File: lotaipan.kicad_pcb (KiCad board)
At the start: 4 copper layers, 71 parts, among them J1 SMA_through, J2 SMA_through, P1 47309-2651_uSD_slot, P2 CONN_01X20, P3 CONN_01X25, P4 USB_OTG, Q1 MOS_N_SGD, U1 RN2483, U2 STM32F405R, U3 MCP1703, U4 MCP73831-2ACI/0T, U5 MIC94091YC6, U6 MIC94091YC6, Y1 12MHz, Y2 32kHz

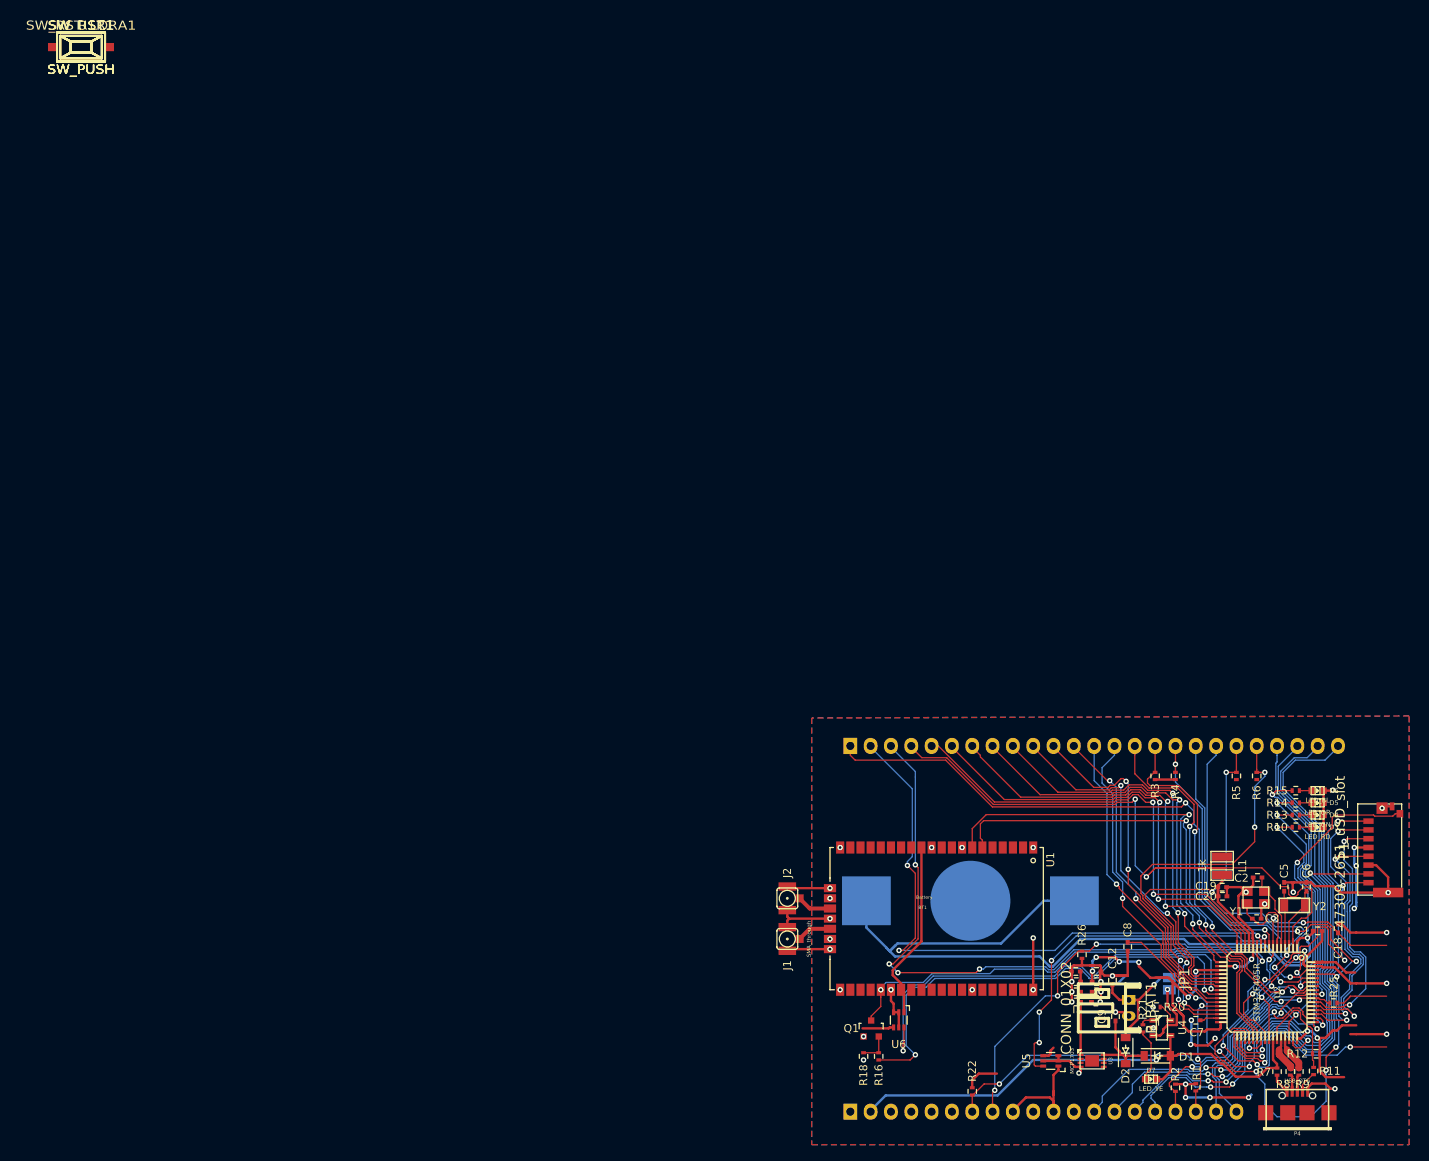
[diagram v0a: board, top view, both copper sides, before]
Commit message: Fixes and images
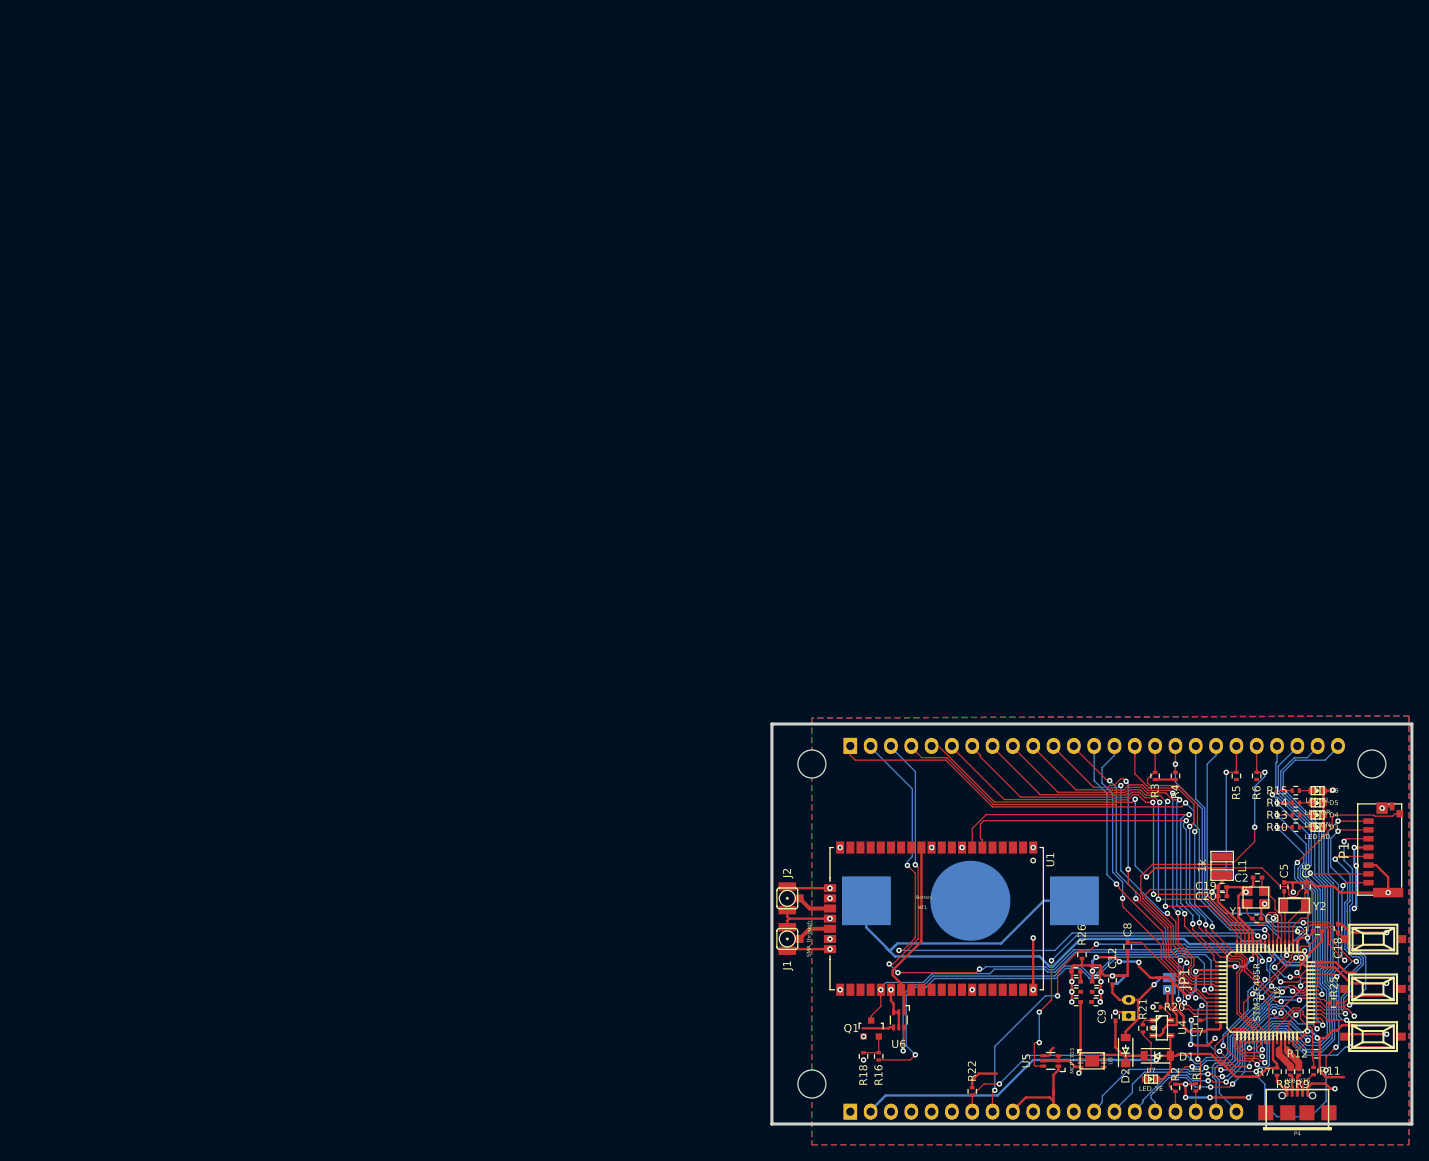
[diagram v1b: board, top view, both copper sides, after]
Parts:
- added REF**: EuroBoard_viertel_Type-I_80mmX50mm_holes, EuroBoard_Outline:EuroBoard_viertel_Type-I_80mmX50mm_holes, F.Cu at (86.4, 134.6)
- P_BAT1: moved to B.Cu
- moved SW_USR1 203.4 mm to (161.5, 123.7)
- moved SW_RST_LORA1 199.9 mm to (161.5, 117.7)
- moved SW_RST1 196.3 mm to (161.5, 111.5)
- turned P_BAT1 to 90 degrees
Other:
- board outline added: 80 x 50 mm
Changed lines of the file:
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@@
   (general
     (links 214)
-    (no_connects 5)
-    (area -7.145 -3.73632 166.012001 138.071333)
+    (no_connects 13)
+    (area 85.95 79.6846 168.64582 140.65626)
     (thickness 1.6)
     (drawings 50)
     (tracks 1879)
     (zones 0)
-    (modules 71)
+    (modules 72)
     (nets 81)
   )
@@
       (effects (font (thickness 0.3048)))
     )
-    (fp_text value 47309-2651_uSD_slot (at 0 -2.2 90) (layer F.SilkS)
+    (fp_text value 47309-2651_uSD_slot (at 0 -2.2 90) (layer F.SilkS) hide
       (effects (font (thickness 0.3048)))
     )
@@
       (effects (font (size 1.27 1.27) (thickness 0.0889)))
     )
-    (fp_text value Jumper_NC_Small (at 0 0 90) (layer B.SilkS)
+    (fp_text value Jumper_NC_Small (at 0 0 90) (layer B.SilkS) hide
       (effects (font (thickness 0.15)) (justify mirror))
     )
@@
       (net 3 VBAT))
   )
-  (module w_conn_jst-ph:s2b-ph-kl (layer Top)
-    (at 130.96 120.10876 270)
+  (module w_conn_jst-ph:s2b-ph-kl (layer Bottom)
+    (at 130.96 120.10876 90)
     (descr "JST PH series connector, S2B-PH-KL")
-    (fp_text reference P_BAT1 (at 0 -2.79908 270) (layer F.SilkS)
-      (effects (font (thickness 0.3048)))
-    )
-    (fp_text value CONN_01X02 (at 0 7.80034 270) (layer F.SilkS)
-      (effects (font (thickness 0.3048)))
-    )
-    (fp_line (start -1.30048 4.09956) (end -1.30048 6.2992) (layer F.SilkS) (width 0.381))
-    (fp_line (start -1.30048 6.2992) (end -1.6002 6.2992) (layer F.SilkS) (width 0.381))
-    (fp_line (start -1.6002 6.2992) (end -1.6002 4.09956) (layer F.SilkS) (width 0.381))
-    (fp_line (start 0.50038 1.99898) (end 0.50038 6.2992) (layer F.SilkS) (width 0.381))
-    (fp_line (start -0.50038 1.99898) (end -0.50038 6.2992) (layer F.SilkS) (width 0.381))
-    (fp_line (start 0.50038 1.99898) (end -0.50038 1.99898) (layer F.SilkS) (width 0.381))
-    (fp_line (start 1.29794 4.09956) (end 1.29794 2.49936) (layer F.SilkS) (width 0.381))
-    (fp_line (start 2.2987 4.09956) (end 1.29794 4.09956) (layer F.SilkS) (width 0.381))
-    (fp_line (start 2.2987 2.49936) (end 2.2987 4.09956) (layer F.SilkS) (width 0.381))
-    (fp_line (start 1.29794 2.49936) (end 2.2987 2.49936) (layer F.SilkS) (width 0.381))
-    (fp_line (start -2.30124 2.49936) (end -1.30048 2.49936) (layer F.SilkS) (width 0.381))
-    (fp_line (start -1.30048 2.49936) (end -1.30048 4.09956) (layer F.SilkS) (width 0.381))
-    (fp_line (start -1.30048 4.09956) (end -2.30124 4.09956) (layer F.SilkS) (width 0.381))
-    (fp_line (start -2.30124 4.09956) (end -2.30124 2.49936) (layer F.SilkS) (width 0.381))
-    (fp_line (start 2.99974 0.39878) (end -2.99974 0.39878) (layer F.SilkS) (width 0.381))
-    (fp_line (start 2.79908 -1.39954) (end 2.79908 0.39878) (layer F.SilkS) (width 0.381))
-    (fp_line (start -2.79908 -1.39954) (end -2.79908 0.39878) (layer F.SilkS) (width 0.381))
-    (fp_line (start -2.99974 6.2992) (end 2.99974 6.2992) (layer F.SilkS) (width 0.381))
-    (fp_line (start 2.99974 6.2992) (end 2.99974 -1.39954) (layer F.SilkS) (width 0.381))
-    (fp_line (start 2.99974 -1.39954) (end 2.60096 -1.39954) (layer F.SilkS) (width 0.381))
-    (fp_line (start 2.60096 -1.39954) (end 2.60096 0.39878) (layer F.SilkS) (width 0.381))
-    (fp_line (start -2.60096 0.39878) (end -2.60096 -1.39954) (layer F.SilkS) (width 0.381))
-    (fp_line (start -2.60096 -1.39954) (end -2.99974 -1.39954) (layer F.SilkS) (width 0.381))
-    (fp_line (start -2.99974 -1.39954) (end -2.99974 6.2992) (layer F.SilkS) (width 0.381))
-    (pad 1 thru_hole rect (at -1.00076 0 270) (size 1.19888 1.69926) (drill 0.70104) (layers *.Cu *.Mask F.SilkS)
+    (fp_text reference P_BAT1 (at 0 2.79908 90) (layer B.SilkS) hide
+      (effects (font (thickness 0.3048)) (justify mirror))
+    )
+    (fp_text value CONN_01X02 (at 0 -7.80034 90) (layer B.SilkS) hide
+      (effects (font (thickness 0.3048)) (justify mirror))
+    )
+    (fp_line (start -1.30048 -4.09956) (end -1.30048 -6.2992) (layer B.SilkS) (width 0.381))
+    (fp_line (start -1.30048 -6.2992) (end -1.6002 -6.2992) (layer B.SilkS) (width 0.381))
+    (fp_line (start -1.6002 -6.2992) (end -1.6002 -4.09956) (layer B.SilkS) (width 0.381))
+    (fp_line (start 0.50038 -1.99898) (end 0.50038 -6.2992) (layer B.SilkS) (width 0.381))
+    (fp_line (start -0.50038 -1.99898) (end -0.50038 -6.2992) (layer B.SilkS) (width 0.381))
+    (fp_line (start 0.50038 -1.99898) (end -0.50038 -1.99898) (layer B.SilkS) (width 0.381))
+    (fp_line (start 1.29794 -4.09956) (end 1.29794 -2.49936) (layer B.SilkS) (width 0.381))
+    (fp_line (start 2.2987 -4.09956) (end 1.29794 -4.09956) (layer B.SilkS) (width 0.381))
+    (fp_line (start 2.2987 -2.49936) (end 2.2987 -4.09956) (layer B.SilkS) (width 0.381))
+    (fp_line (start 1.29794 -2.49936) (end 2.2987 -2.49936) (layer B.SilkS) (width 0.381))
+    (fp_line (start -2.30124 -2.49936) (end -1.30048 -2.49936) (layer B.SilkS) (width 0.381))
+    (fp_line (start -1.30048 -2.49936) (end -1.30048 -4.09956) (layer B.SilkS) (width 0.381))
+    (fp_line (start -1.30048 -4.09956) (end -2.30124 -4.09956) (layer B.SilkS) (width 0.381))
+    (fp_line (start -2.30124 -4.09956) (end -2.30124 -2.49936) (layer B.SilkS) (width 0.381))
+    (fp_line (start 2.99974 -0.39878) (end -2.99974 -0.39878) (layer B.SilkS) (width 0.381))
+    (fp_line (start 2.79908 1.39954) (end 2.79908 -0.39878) (layer B.SilkS) (width 0.381))
+    (fp_line (start -2.79908 1.39954) (end -2.79908 -0.39878) (layer B.SilkS) (width 0.381))
+    (fp_line (start -2.99974 -6.2992) (end 2.99974 -6.2992) (layer B.SilkS) (width 0.381))
+    (fp_line (start 2.99974 -6.2992) (end 2.99974 1.39954) (layer B.SilkS) (width 0.381))
+    (fp_line (start 2.99974 1.39954) (end 2.60096 1.39954) (layer B.SilkS) (width 0.381))
+    (fp_line (start 2.60096 1.39954) (end 2.60096 -0.39878) (layer B.SilkS) (width 0.381))
+    (fp_line (start -2.60096 -0.39878) (end -2.60096 1.39954) (layer B.SilkS) (width 0.381))
+    (fp_line (start -2.60096 1.39954) (end -2.99974 1.39954) (layer B.SilkS) (width 0.381))
+    (fp_line (start -2.99974 1.39954) (end -2.99974 -6.2992) (layer B.SilkS) (width 0.381))
+    (pad 1 thru_hole rect (at -1.00076 0 90) (size 1.19888 1.69926) (drill 0.70104) (layers *.Cu *.Mask B.SilkS)
       (net 3 VBAT))
-    (pad 2 thru_hole oval (at 1.00076 0 270) (size 1.19888 1.69926) (drill 0.70104) (layers *.Cu *.Mask F.SilkS)
+    (pad 2 thru_hole oval (at 1.00076 0 90) (size 1.19888 1.69926) (drill 0.70104) (layers *.Cu *.Mask B.SilkS)
       (net 2 GND))
     (model walter/conn_jst-ph/s2b-ph-kl.wrl
@@
   )
   (module w_switch:smd_push (layer Top)
-    (at 0 0)
+    (at 161.544 111.506)
     (descr "SMD Pushbutton")
     (autoplace_cost180 10)
-    (fp_text reference SW_RST1 (at 0 -2.70002) (layer F.SilkS)
+    (fp_text reference SW_RST1 (at 0 -2.70002) (layer F.SilkS) hide
       (effects (font (size 1.143 1.27) (thickness 0.1524)))
     )
-    (fp_text value SW_PUSH (at 0 2.79908) (layer F.SilkS)
+    (fp_text value SW_PUSH (at 0 2.79908) (layer F.SilkS) hide
       (effects (font (size 1.143 1.27) (thickness 0.1524)))
     )
@@
   )
   (module w_switch:smd_push (layer Top)
-    (at 0 0)
+    (at 161.50082 117.729)
     (descr "SMD Pushbutton")
     (autoplace_cost180 10)
-    (fp_text reference SW_RST_LORA1 (at 0 -2.70002) (layer F.SilkS)
+    (fp_text reference SW_RST_LORA1 (at 0 -2.70002) (layer F.SilkS) hide
       (effects (font (size 1.143 1.27) (thickness 0.1524)))
     )
-    (fp_text value SW_PUSH (at 0 2.79908) (layer F.SilkS)
+    (fp_text value SW_PUSH (at 0 2.79908) (layer F.SilkS) hide
       (effects (font (size 1.143 1.27) (thickness 0.1524)))
     )
@@
   )
   (module w_switch:smd_push (layer Top)
-    (at 0 0)
+    (at 161.50082 123.698)
     (descr "SMD Pushbutton")
     (autoplace_cost180 10)
-    (fp_text reference SW_USR1 (at 0 -2.70002) (layer F.SilkS)
+    (fp_text reference SW_USR1 (at 0 -2.70002) (layer F.SilkS) hide
       (effects (font (size 1.143 1.27) (thickness 0.1524)))
     )
-    (fp_text value SW_PUSH (at 0 2.79908) (layer F.SilkS)
+    (fp_text value SW_PUSH (at 0 2.79908) (layer F.SilkS) hide
       (effects (font (size 1.143 1.27) (thickness 0.1524)))
     )
@@
     )
   )
+  (module EuroBoard_Outline:EuroBoard_viertel_Type-I_80mmX50mm_holes (layer Top)
+    (at 86.36 134.62)
+    (descr "Outline, Eurocard 1/4, Type I,  80x50mm, with holes 3,5mm,")
+    (tags "Outline, Eurocard 1/4, Type I, 80x50mm, with holes 3,5mm,")
+    (fp_text reference REF** (at 41.00068 -54.0004) (layer F.SilkS) hide
+      (effects (font (size 1 1) (thickness 0.15)))
+    )
+    (fp_text value EuroBoard_viertel_Type-I_80mmX50mm_holes (at 41.9989 5.00126) (layer F.Fab)
+      (effects (font (size 1 1) (thickness 0.15)))
+    )
+    (fp_line (start 0 0) (end 0 -49.9999) (layer Edge.Cuts) (width 0.381))
+    (fp_line (start 0 -49.9999) (end 79.99984 -49.9999) (layer Edge.Cuts) (width 0.381))
+    (fp_line (start 79.99984 -49.9999) (end 79.99984 0) (layer Edge.Cuts) (width 0.381))
+    (fp_line (start 79.99984 0) (end 0 0) (layer Edge.Cuts) (width 0.381))
+    (pad "" np_thru_hole circle (at 5.00126 -5.00126) (size 3.50012 3.50012) (drill 3.50012) (layers *.Cu *.Mask F.SilkS))
+    (pad "" np_thru_hole circle (at 5.00126 -45.00118) (size 3.50012 3.50012) (drill 3.50012) (layers *.Cu *.Mask F.SilkS))
+    (pad "" np_thru_hole circle (at 75.00112 -45.00118) (size 3.50012 3.50012) (drill 3.50012) (layers *.Cu *.Mask F.SilkS))
+    (pad "" np_thru_hole circle (at 75.00112 -5.00126) (size 3.50012 3.50012) (drill 3.50012) (layers *.Cu *.Mask F.SilkS))
+  )
   (gr_text "loTaipan V 0.1.0\nHacked in Switzerland" (at 149.375 96.502 90) (layer B.SilkS)
